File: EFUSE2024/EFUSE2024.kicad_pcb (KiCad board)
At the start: 2 copper layers, 34 parts, among them J1 Conn_01x03_Pin, Q1 CSD19537Q3, Q2 BSS138, U1 TPS26630RGE, U2 TPS26630RGE, U3 TPS26630RGE, U7 TPS26630RGE

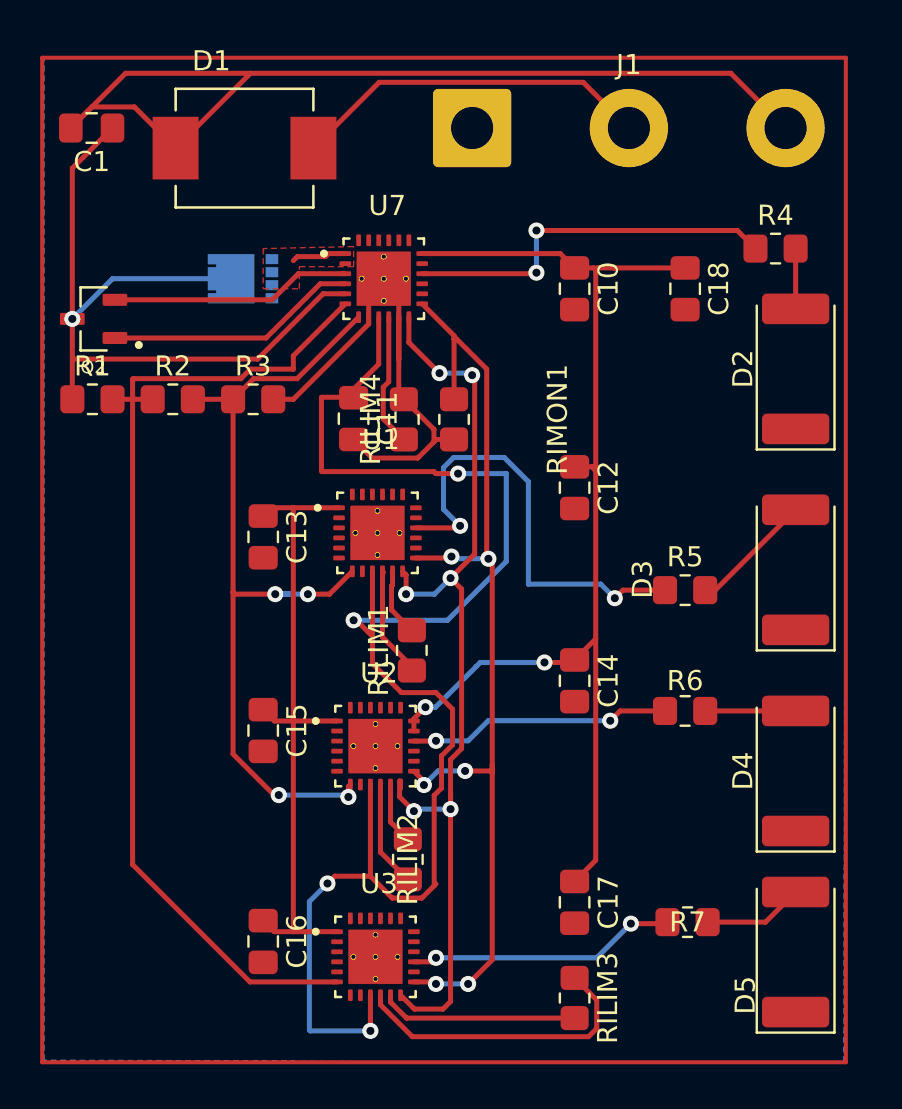
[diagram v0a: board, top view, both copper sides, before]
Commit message: fixed up PCB
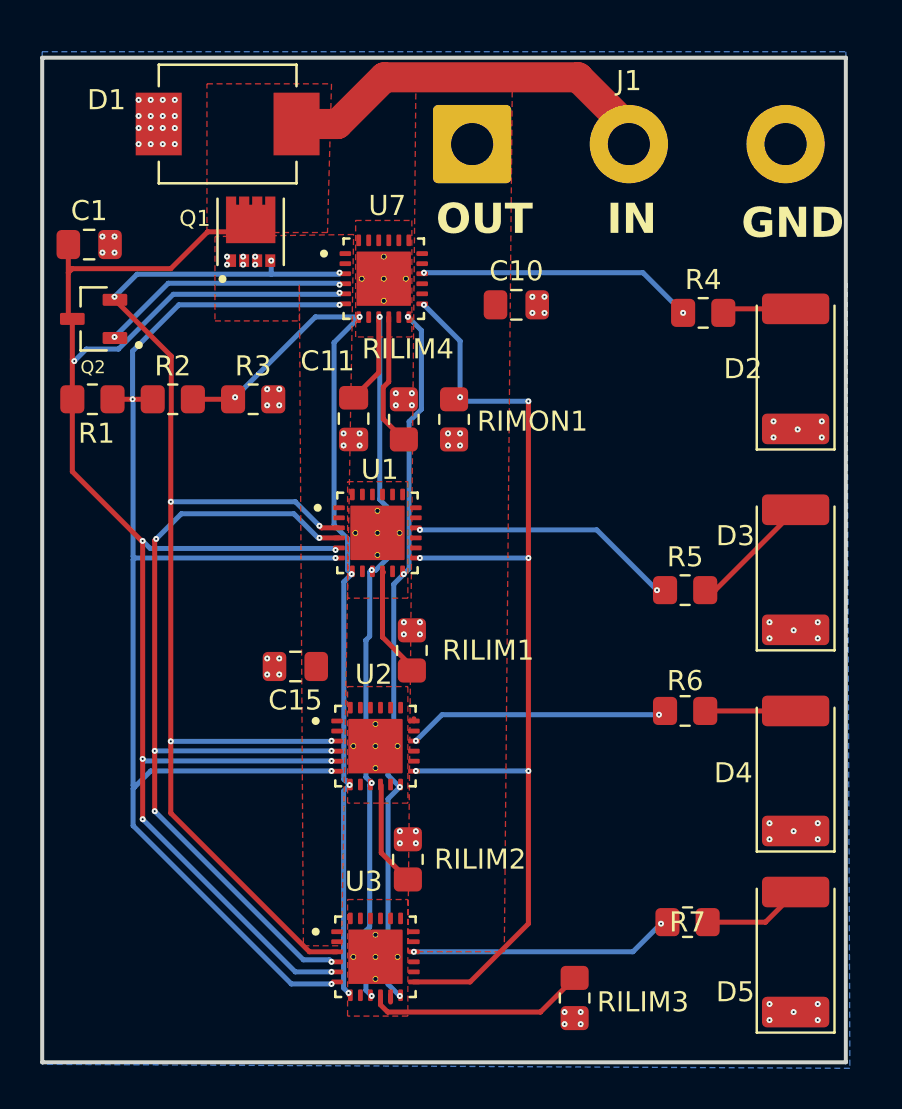
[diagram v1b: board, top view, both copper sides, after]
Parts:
- removed C12, C13, C14, C16, C17, C18: 0.1uF, Capacitor_SMD:C_0805_2012Metric_Pad1.18x1.45mm_HandSolder
- Q1: moved to F.Cu
- moved C1 5.80 mm to (94.3, 78.8), turned to 0 degrees
- moved R4 4.82 mm to (124.9, 82.2)
- moved C15 3.57 mm to (104.6, 99.8), turned to 180 degrees
- moved C10 3.01 mm to (115.6, 81.8), turned to 0 degrees
- moved Q1 2.36 mm to (102.4, 78.2), turned to 90 degrees
- moved D1 1.46 mm to (101.2, 72.8)
- moved J1 0.80 mm to (113.4, 73.8)
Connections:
- C15 pad 1: Net-(C13-Pad1) -> Net-(U1-DRV)
- Q1 pad 1: Net-(C13-Pad1) -> Net-(U1-DRV)
- Q1 pad 2: Net-(C13-Pad1) -> Net-(U1-DRV)
- Q1 pad 3: Net-(C13-Pad1) -> Net-(U1-DRV)
- Q1 pad 4: Net-(U7-B_GATE) -> Net-(U1-B_GATE)
- Q2 pad 1: Net-(U7-DRV) -> Net-(U1-DRV)
- Q2 pad 2: Net-(U7-B_GATE) -> Net-(U1-B_GATE)
- R7 pad 1: Net-(U3-PGTH) -> Net-(U3-PGOOD)
- U1 pad 1: Net-(C13-Pad1) -> Net-(U1-DRV)
- U1 pad 2: Net-(C13-Pad1) -> Net-(U1-DRV)
- U1 pad 3: unconnected-(U1-B_GATE-Pad3) -> Net-(U1-B_GATE)
- U1 pad 4: unconnected-(U1-DRV-Pad4) -> Net-(U1-DRV)
- U2 pad 1: Net-(C13-Pad1) -> Net-(U1-DRV)
- U2 pad 2: Net-(C13-Pad1) -> Net-(U1-DRV)
- U2 pad 3: unconnected-(U2-B_GATE-Pad3) -> Net-(U1-B_GATE)
- U2 pad 4: unconnected-(U2-DRV-Pad4) -> Net-(U1-DRV)
- U3 pad 1: Net-(C13-Pad1) -> Net-(U1-DRV)
- U3 pad 15: Net-(U3-PGTH) -> unconnected-(U3-PGTH-Pad15)
- U3 pad 16: unconnected-(U3-PGOOD-Pad16) -> Net-(U3-PGOOD)
- U3 pad 2: Net-(C13-Pad1) -> Net-(U1-DRV)
- U3 pad 3: unconnected-(U3-B_GATE-Pad3) -> Net-(U1-B_GATE)
- U3 pad 4: unconnected-(U3-DRV-Pad4) -> Net-(U1-DRV)
- U3 pad 7: unconnected-(U3-OVP-Pad7) -> Net-(U1-OVP)
- U7 pad 1: Net-(C13-Pad1) -> Net-(U1-DRV)
- U7 pad 2: Net-(C13-Pad1) -> Net-(U1-DRV)
- U7 pad 3: Net-(U7-B_GATE) -> Net-(U1-B_GATE)
- U7 pad 4: Net-(U7-DRV) -> Net-(U1-DRV)
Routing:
- net GND: track 90.7 -> 0.34 mm, vias 0 -> 76
- net Net-(U1-B_GATE): track 0.00 -> 67.1 mm, vias 0 -> 7
- net Net-(U1-DRV): track 0.00 -> 56.7 mm, vias 0 -> 14
- net Net-(J1-Pin_1): track 57.1 -> 0.97 mm, vias 2 -> 0
- net Net-(J1-Pin_2): track 56.9 -> 105.7 mm, vias 1 -> 8
- net Net-(U1-dVdT): track 75.7 -> 39.4 mm
- net Net-(C13-Pad1): track 35.6 -> 0.00 mm
- net Net-(U1-UVLO): track 51.5 -> 70.3 mm, vias 0 -> 5
- net Net-(U3-PGTH): track 13.4 -> 0.00 mm, vias 2 -> 0
- net Net-(U1-~{SHDN}): track 48.6 -> 35.5 mm, vias 6 -> 4
- net Net-(U3-PGOOD): track 0.00 -> 13.0 mm, vias 0 -> 2
- net Net-(U7-DRV): track 12.6 -> 0.00 mm
- net Net-(U7-B_GATE): track 12.1 -> 0.00 mm
- net Net-(U1-PGOOD): track 22.8 -> 13.0 mm
- net Net-(U7-PGOOD): track 19.1 -> 13.7 mm
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- added copper zone on F.Cu, net GND
- added copper zone on F.Cu, net Net-(J1-Pin_1)
- added copper zone on F.Cu, net Net-(J1-Pin_2)
- added copper zone on F.Cu, net Net-(U1-DRV)
- removed copper zone on F.Cu, net (none)
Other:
- board outline added: 40 x 50 mm
- board text added: "GND"
- board text added: "IN"
- board text added: "OUT"
